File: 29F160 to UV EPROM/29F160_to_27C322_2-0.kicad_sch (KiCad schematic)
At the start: 12 parts, among them U1 27C322, U2 29F160, U3 29F160, U4 74LS139

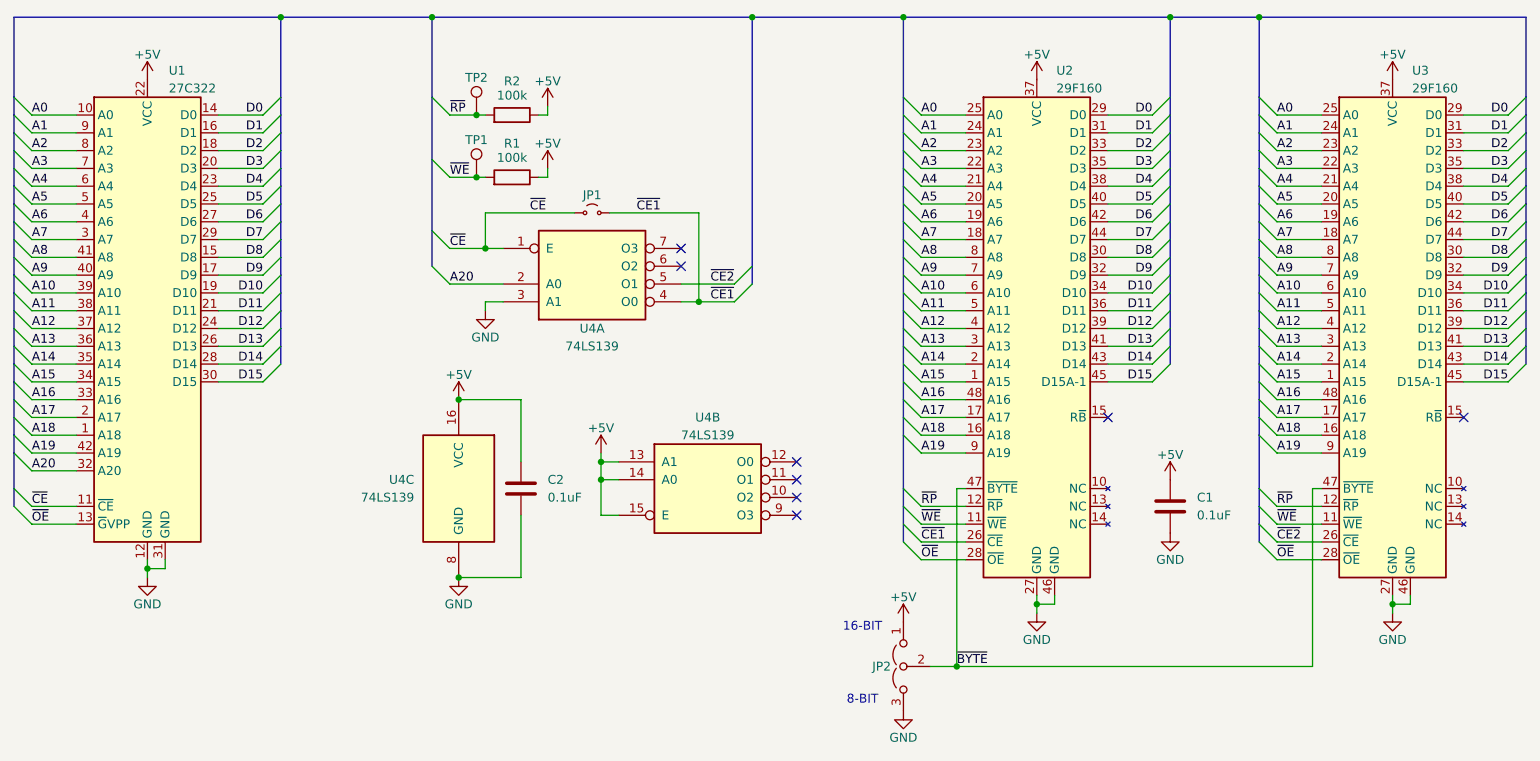
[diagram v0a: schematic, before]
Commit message: Add files via upload
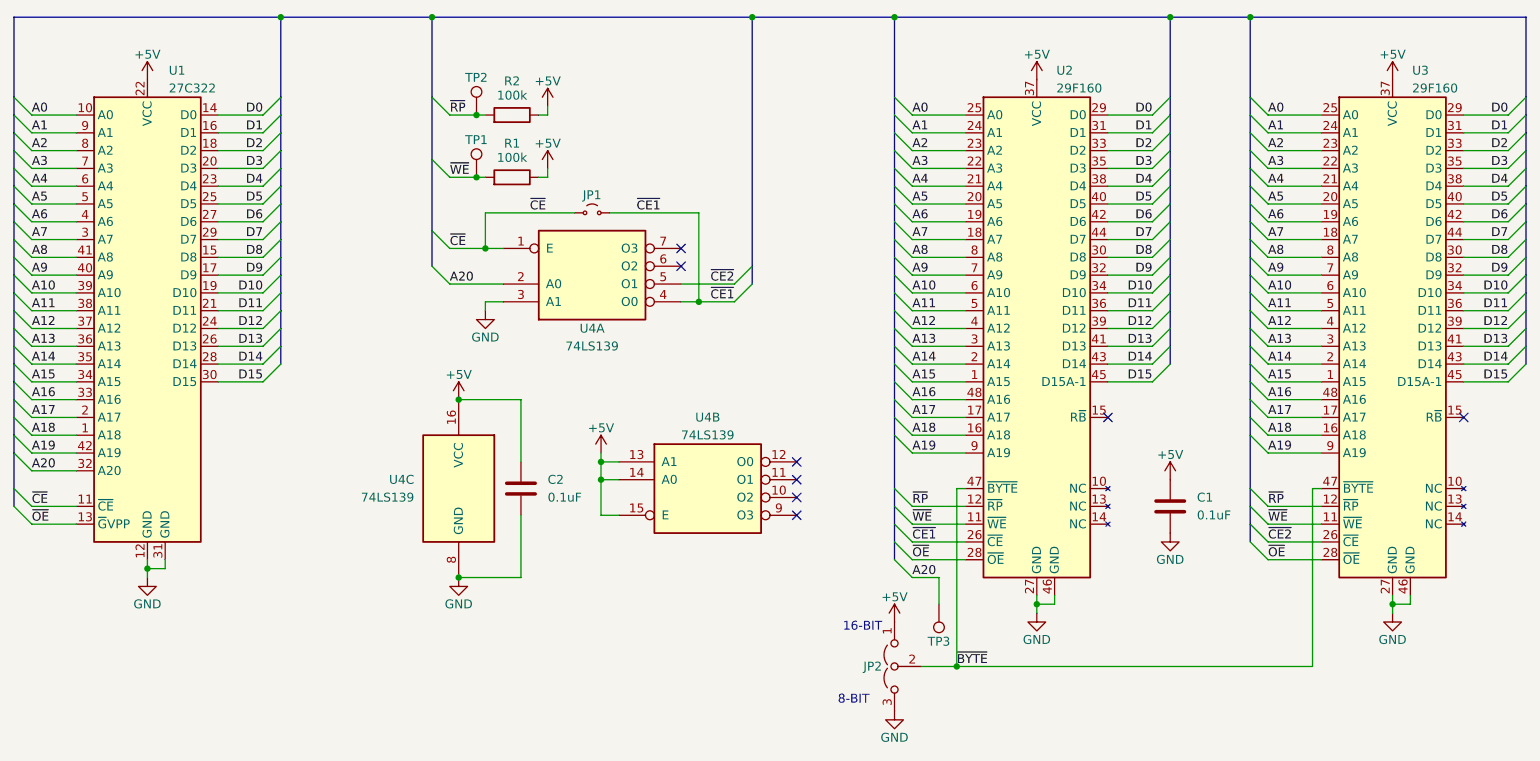
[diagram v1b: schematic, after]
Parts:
- added TP3: TPB1,27, TestPoint:TestPoint_Pad_1.0x1.0mm, symbol Connector:TestPoint
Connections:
- net A20: now also TP3.1
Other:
- moved on the sheet: JP2
